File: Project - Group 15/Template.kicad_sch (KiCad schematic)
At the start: 5 parts, among them J1 RJ45

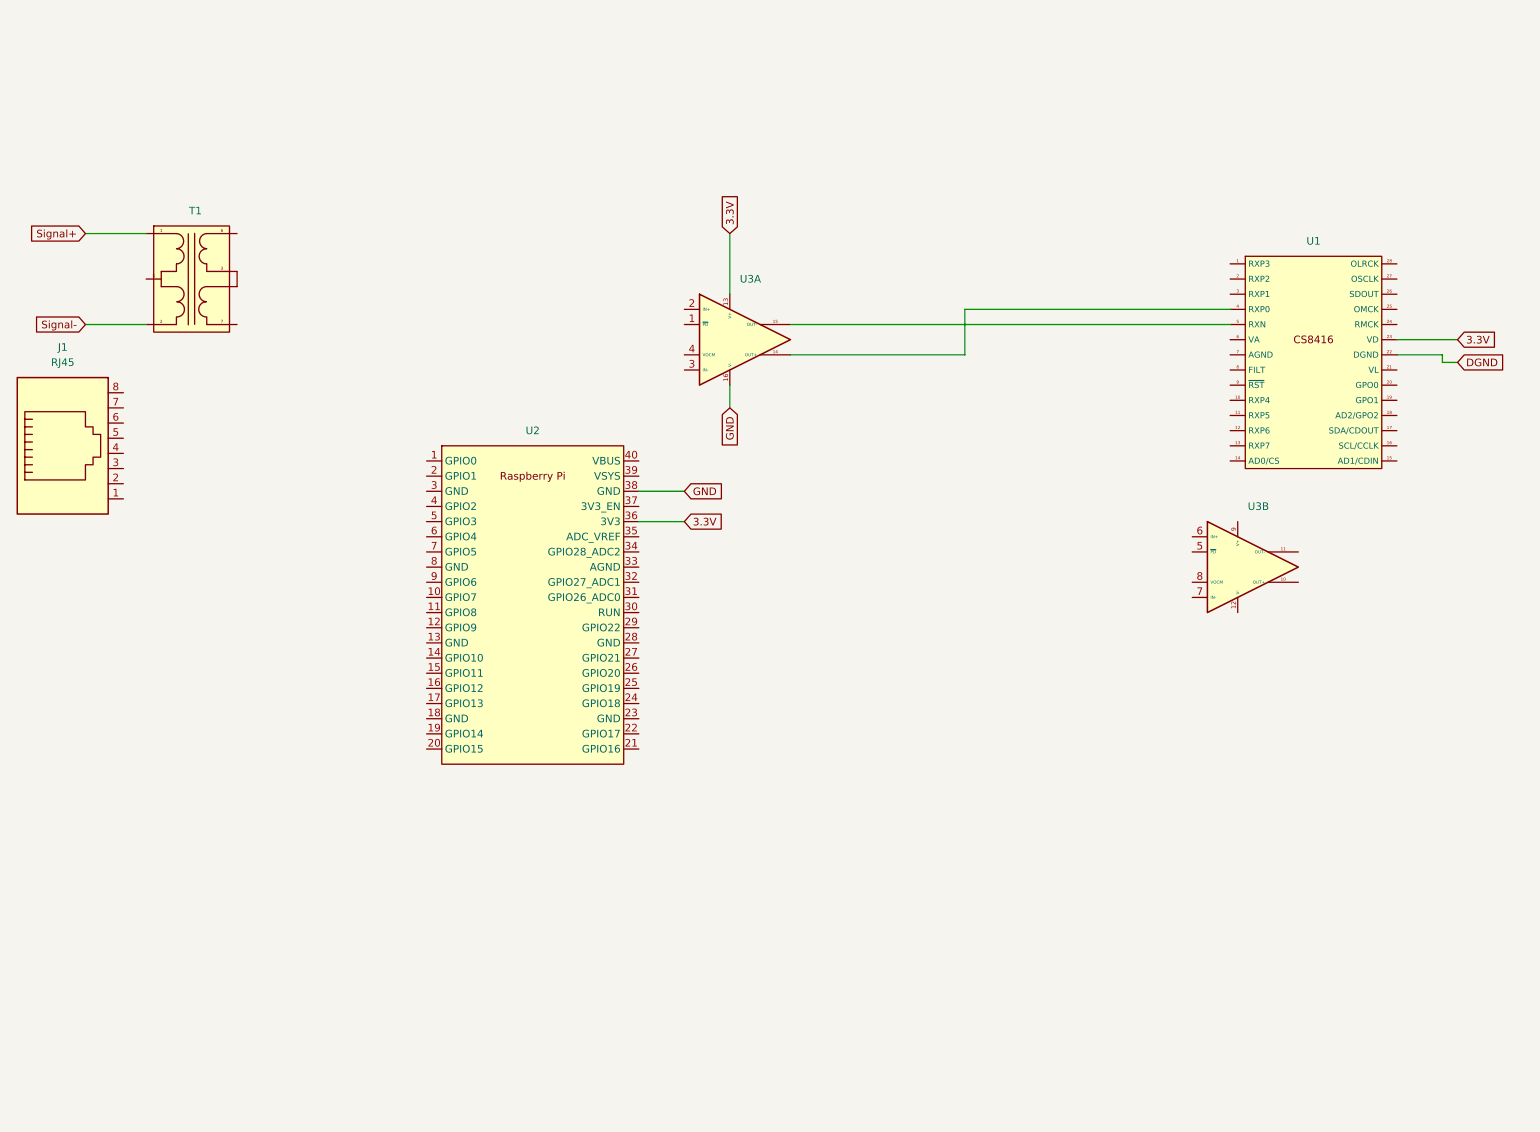
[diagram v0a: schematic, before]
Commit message: mar 9
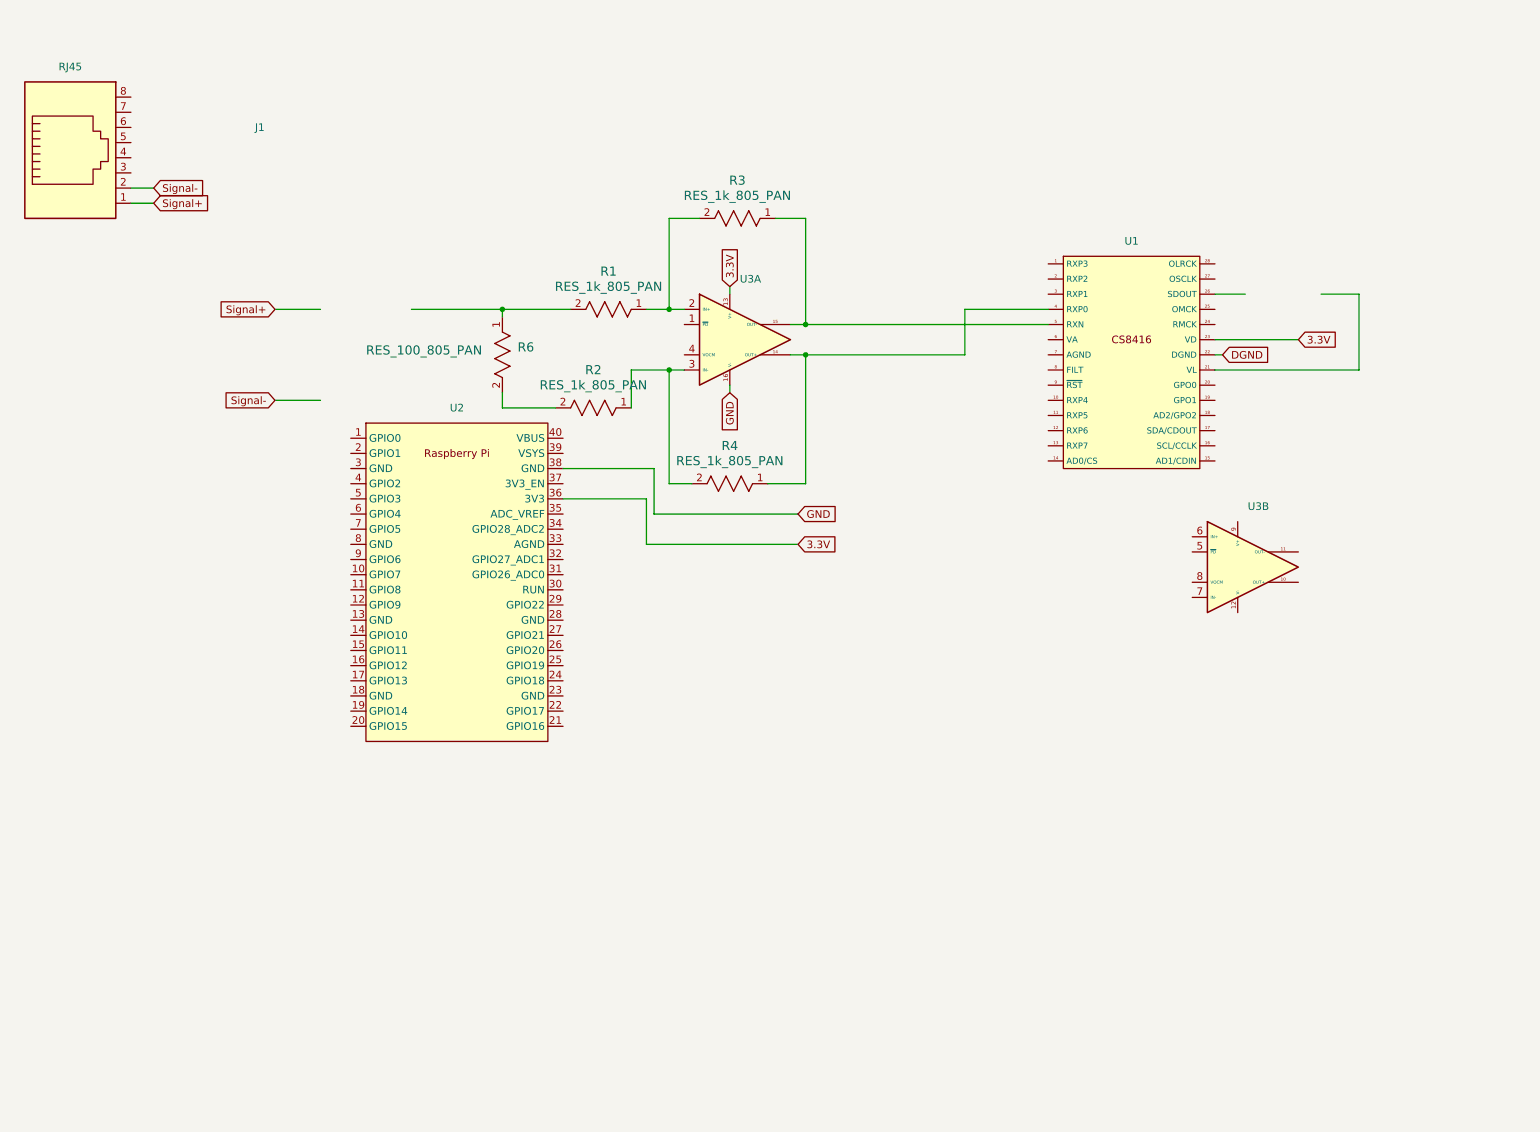
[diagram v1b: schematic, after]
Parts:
- removed T1: ~, 491_Footprints:SM453230-181N7Y, symbol 491_Symbols:SM453230-181N7Y
- added R1, R2, R3, R4: RES_1k_805_PAN, RC0402N_PAN, symbol 491_Symbols:RES_1k_805_PAN
- added R6: RES_100_805_PAN, RES_ERJ6B_0805_PAN, symbol 491_Symbols:RES_100_805_PAN
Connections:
- net Signal+: now also J1.1
- net Signal-: now also J1.2
- net at U1.4 (RXP0), U3.14 (OUT+): now also R4.1
- net at U1.5 (RXN), U3.15 (OUT-): now also R3.1
- net at U3.2 (IN+): now also R1.1, R3.2
- net at U3.3 (IN-): now also R2.1, R4.2
- new net: R1.2, R6.1
- new net: R2.2, R6.2
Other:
- moved on the sheet: J1, U1, U2

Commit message: Group 15
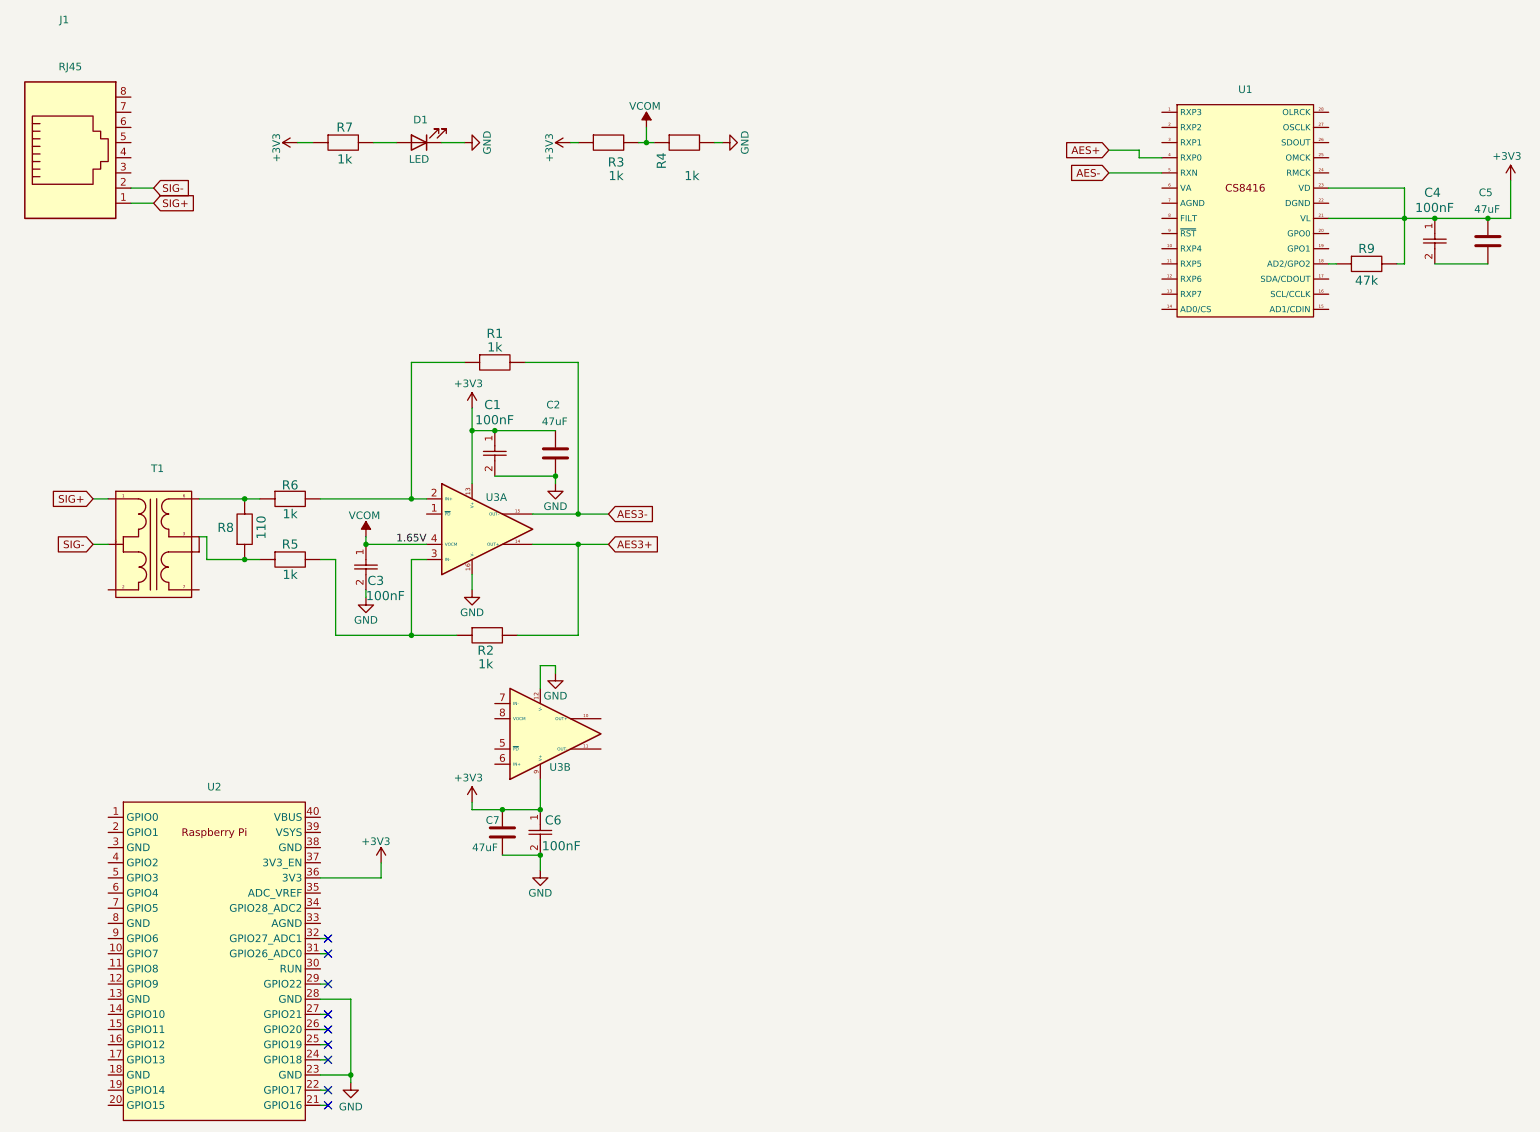
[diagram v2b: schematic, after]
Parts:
- removed R6: RES_100_805_PAN, RES_ERJ6B_0805_PAN, symbol 491_Symbols:RES_100_805_PAN
- added C1, C3, C4, C6: 100nF, 491_Footprints:CAP_CER_100nF_SAM, symbol 491_Symbols:CAP_CER_100nF_SAM
- added C2, C5, C7: 47uF, symbol Device:C
- added D1: LED, symbol Device:LED
- added R5, R6, R7: 1k, 491_Footprints:RES_1k_805_PAN, symbol 491_Symbols:RES_1k_805_PAN
- added R8: 110, 491_Footprints:RES_110_805_PAN, symbol 491_Symbols:RES_110_805_PAN
- added R9: 47k, 491_Footprints:RES_47k_805_PAN, symbol 491_Symbols:RES_47k_805_PAN
- added T1: ~, 491_Footprints:SM453230-181N7Y, symbol 491_Symbols:SM453230-181N7Y
- R1, R2, R3, R4: value RES_1k_805_PAN -> 1k; footprint RC0402N_PAN -> 491_Footprints:RES_1k_805_PAN
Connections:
- net 3.3V is gone; now on net +3V3: U1.23 (VD), U2.36 (3V3), U3.13 (V+)
- net GND: now also R4., U2.23 (GND), U2.28 (GND), U3.12 (V-), C1.2, C2.2, C3.2, C6.2, C7.2, D1.1 (K); no longer U2.38 (GND)
- net VCOM: now reaches U3.4 (VOCM)
- net VCOM: now also R3., R4., C3.1
- net at U1.18 (AD2/GPO2): now also R9.
- net +3V3: now reaches U1.21 (VL)
- net +3V3: now also R3., U3.9 (V+), C1.1, C2.1, C4.1, C5.1, C6.1, C7.1, R7., R9.
- net DGND: no longer names the net of U1.22 (DGND)
- net Signal+ renamed SIG+
- net SIG+: now also T1.1
- net Signal- renamed SIG-
- net SIG-: now also T1.5
- new net: D1.2 (A), R7.
- new net: R1., R6., U3.2 (IN+)
- new net: C4.2, C5.2
- new net: R2., R5., U3.3 (IN-)
- new net: R5., R8., T1.3
- new net: R6., R8., T1.6
- new net AES+: U1.4 (RXP0)
- new net AES-: U1.5 (RXN)
- new net AES3+: R2., U3.14 (OUT+)
- new net AES3-: R1., U3.15 (OUT-)
- no-connect marks 0 -> 9
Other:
- moved on the sheet: U1, U2
